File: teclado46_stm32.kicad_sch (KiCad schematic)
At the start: 12 parts, among them J2 78171-0004, U1 XC6206PxxxMR, U2 STM32G474CETx, U4 W25Q128JVS

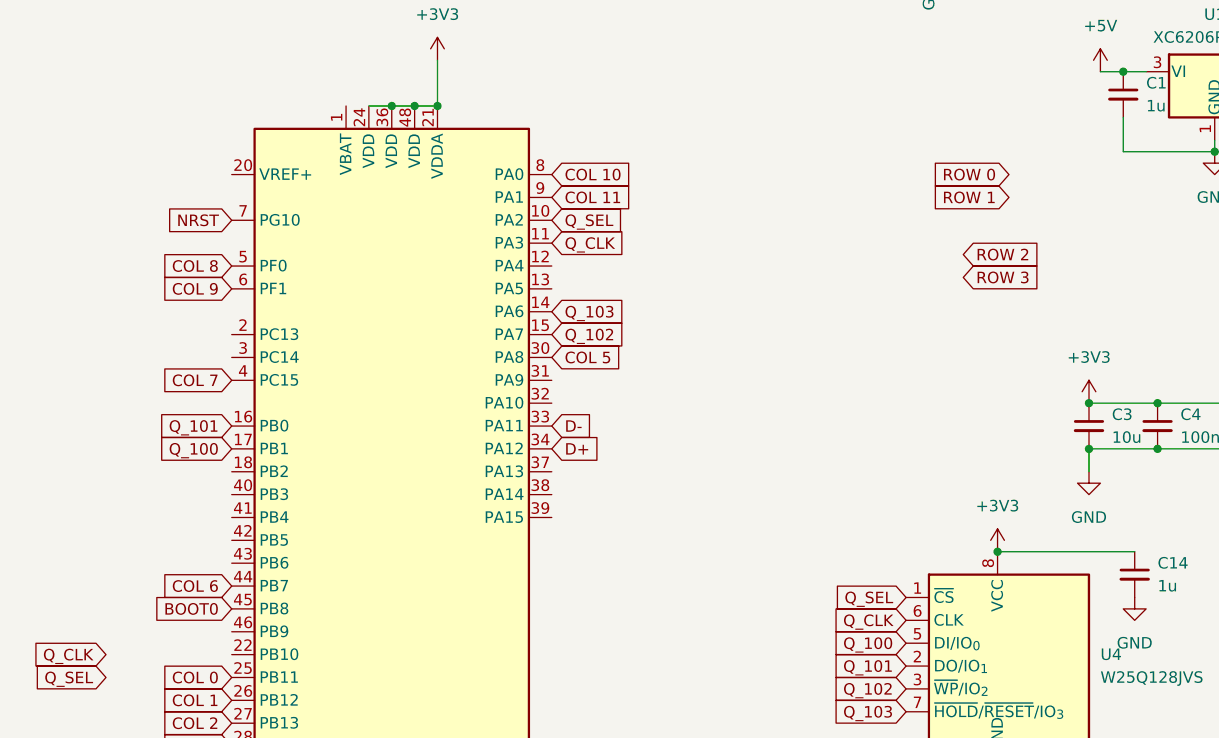
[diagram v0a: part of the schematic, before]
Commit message: chore: routed rows
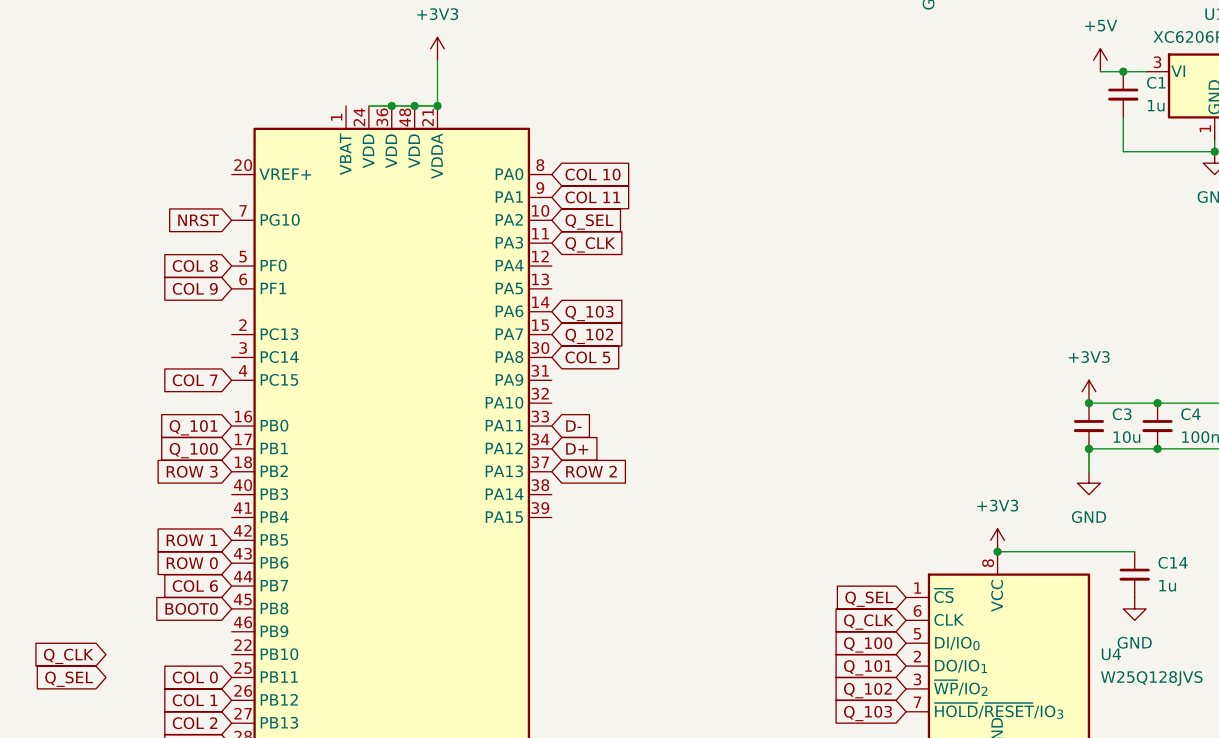
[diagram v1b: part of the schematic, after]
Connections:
- net ROW 0: now also U2.43 (PB6)
- net ROW 1: now also U2.42 (PB5)
- net ROW 2: now also U2.37 (PA13)
- net ROW 3: now also U2.18 (PB2)
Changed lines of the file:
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@@
 	(global_label "ROW 1"
 		(shape input)
-		(at 119.38 113.03 180)
-		(fields_autoplaced yes)
-		(effects
-			(font
-				(size 1.27 1.27)
-			)
-			(justify right)
-		)
-		(property "Intersheetrefs" "${INTERSHEET_REFS}"
-			(at 110.1658 113.03 0)
+		(at 33.02 151.13 180)
+		(fields_autoplaced yes)
+		(effects
+			(font
+				(size 1.27 1.27)
+			)
+			(justify right)
+		)
+		(property "Intersheetrefs" "${INTERSHEET_REFS}"
+			(at 23.8058 151.13 0)
 			(effects
 				(font
@@
 	(global_label "ROW 0"
 		(shape input)
-		(at 119.38 110.49 180)
-		(fields_autoplaced yes)
-		(effects
-			(font
-				(size 1.27 1.27)
-			)
-			(justify right)
-		)
-		(property "Intersheetrefs" "${INTERSHEET_REFS}"
-			(at 110.1658 110.49 0)
+		(at 33.02 153.67 180)
+		(fields_autoplaced yes)
+		(effects
+			(font
+				(size 1.27 1.27)
+			)
+			(justify right)
+		)
+		(property "Intersheetrefs" "${INTERSHEET_REFS}"
+			(at 23.8058 153.67 0)
 			(effects
 				(font
@@
 	(global_label "ROW 2"
 		(shape input)
-		(at 114.3 119.38 0)
-		(fields_autoplaced yes)
-		(effects
-			(font
-				(size 1.27 1.27)
-			)
-			(justify left)
-		)
-		(property "Intersheetrefs" "${INTERSHEET_REFS}"
-			(at 123.5142 119.38 0)
+		(at 68.58 143.51 0)
+		(fields_autoplaced yes)
+		(effects
+			(font
+				(size 1.27 1.27)
+			)
+			(justify left)
+		)
+		(property "Intersheetrefs" "${INTERSHEET_REFS}"
+			(at 77.7942 143.51 0)
 			(effects
 				(font
@@
 	(global_label "ROW 3"
 		(shape input)
-		(at 114.3 121.92 0)
-		(fields_autoplaced yes)
-		(effects
-			(font
-				(size 1.27 1.27)
-			)
-			(justify left)
-		)
-		(property "Intersheetrefs" "${INTERSHEET_REFS}"
-			(at 123.5142 121.92 0)
-			(effects
-				(font
-					(size 1.27 1.27)
-				)
-				(justify left)
-				(hide yes)
-			)
+		(at 33.02 143.51 180)
+		(fields_autoplaced yes)
+		(effects
+			(font
+				(size 1.27 1.27)
+			)
+			(justify right)
+		)
+		(property "Intersheetrefs" "${INTERSHEET_REFS}"
+			(at 23.8058 143.51 0)
+			(effects
+				(font
+					(size 1.27 1.27)
+				)
+				(justify right)
+				(hide yes)
+			)
